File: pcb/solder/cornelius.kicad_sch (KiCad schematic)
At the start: 116 parts, among them J1 AVR-ISP-6, SW1 SW_Push, U1 ATmega32U4-MU, U2 PRTR5V0U2X, Y1 16MHz

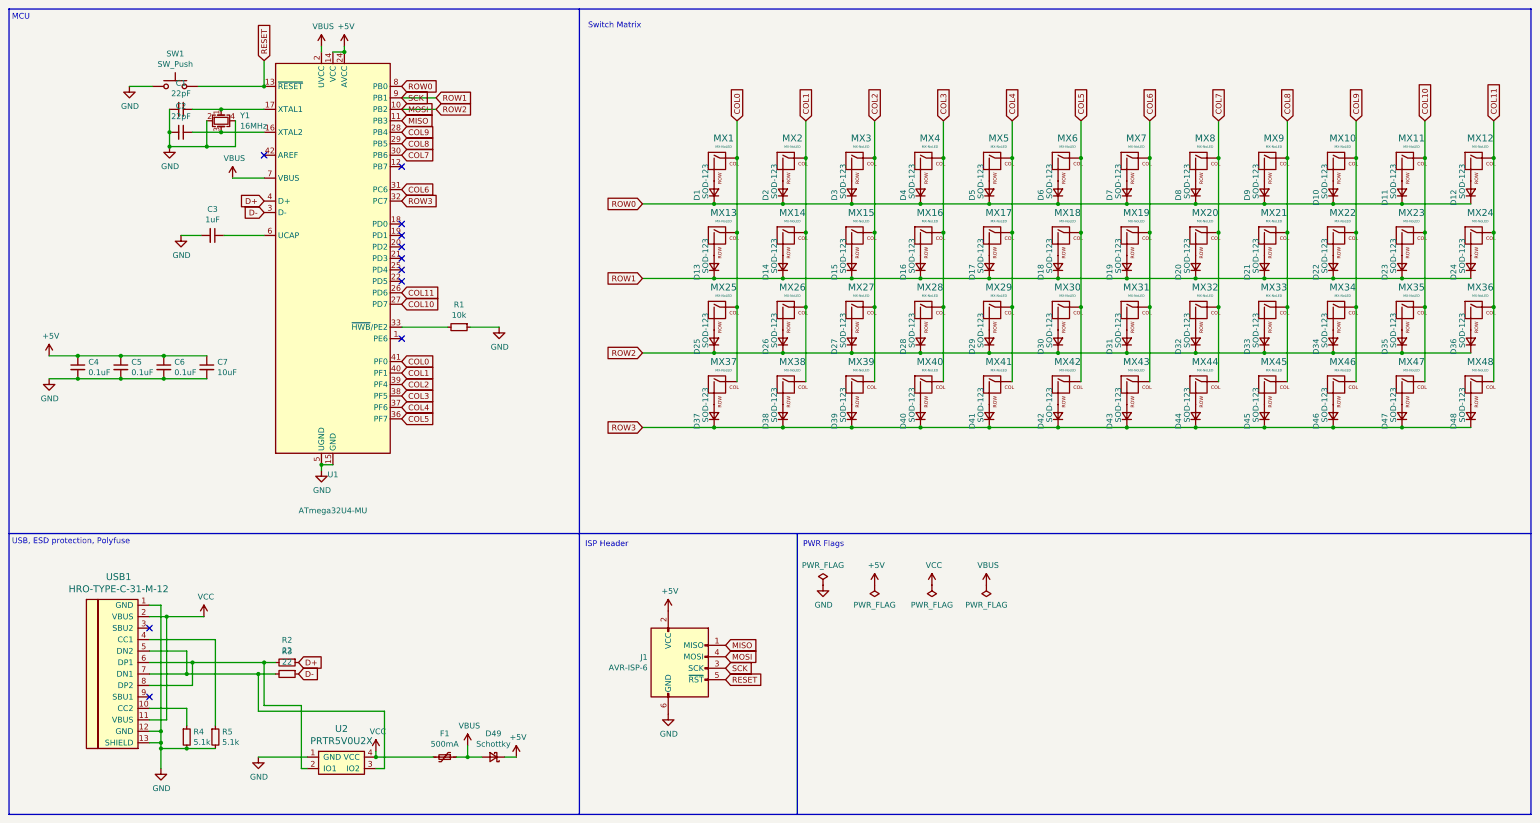
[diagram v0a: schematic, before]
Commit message: Add solder pcb
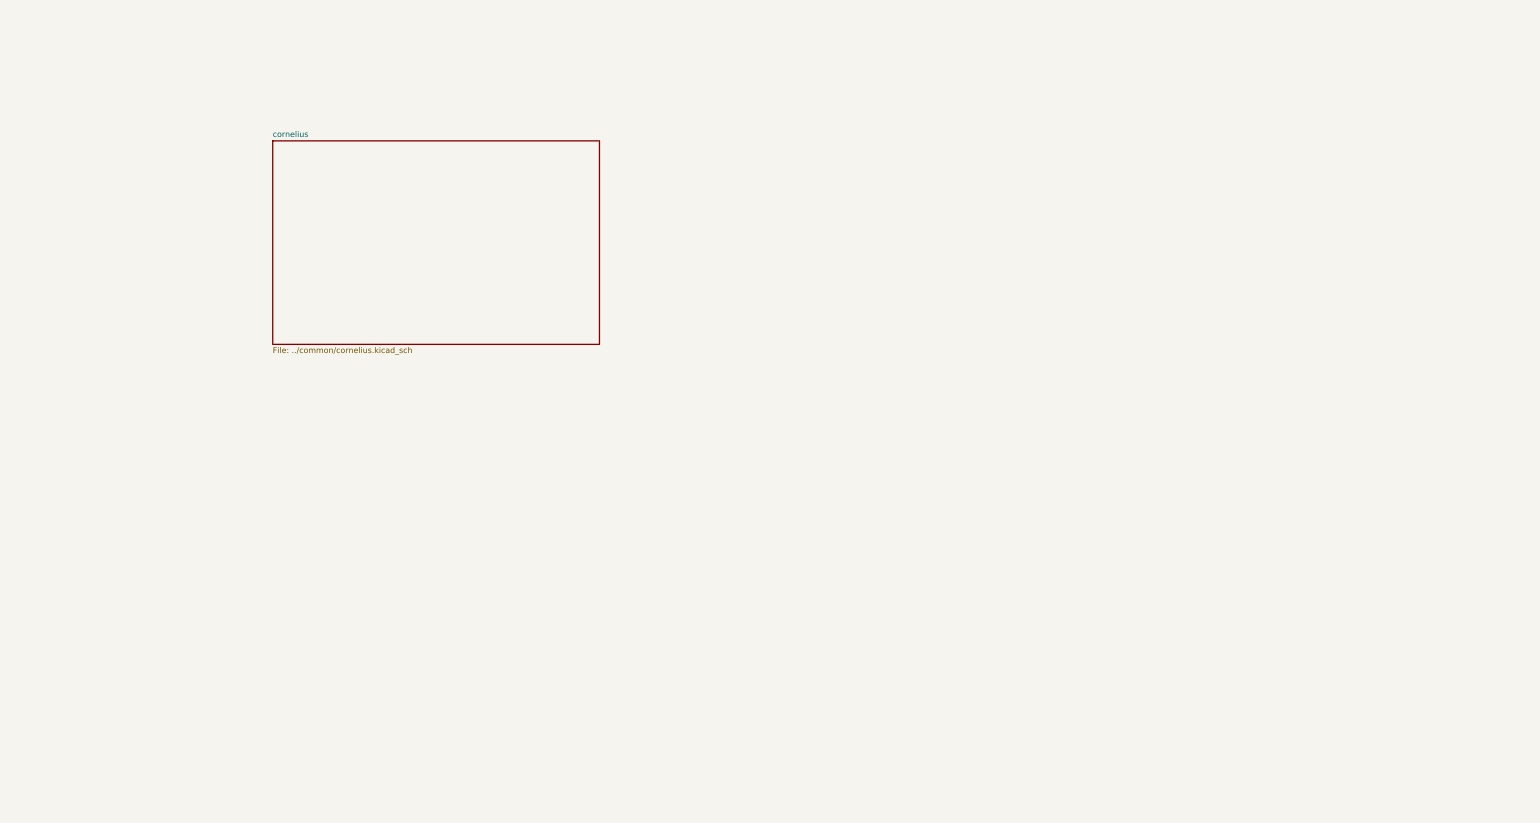
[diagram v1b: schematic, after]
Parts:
- removed C1, C2: 22pF, Capacitor_SMD:C_0603_1608Metric, symbol Device:C_Small
- removed C3: 1uF, Capacitor_SMD:C_0603_1608Metric, symbol Device:C_Small
- removed C4, C5, C6: 0.1uF, Capacitor_SMD:C_0603_1608Metric, symbol Device:C_Small
- removed C7: 10uF, Capacitor_SMD:C_0603_1608Metric, symbol Device:C_Small
- removed D1, D10, D11, D12, D13, D14, D15, D16, D17, D18, D19, D2, D20, D21, D22, D23, D24, D25, D26, D27, D28, D29, D3, D30, D31, D32, D33, D34, D35, D36, D37, D38, D39, D4, D40, D41, D42, D43, D44, D45, D46, D47, D48, D5, D6, D7, D8, D9: SOD-123, Diode_SMD:D_SOD-123, symbol Device:D_Small
- removed D49: Schottky, Diode_SMD:D_SOD-123, symbol Device:D_Schottky_Small
- removed F1: 500mA, Fuse:Fuse_1206_3216Metric, symbol Device:Polyfuse_Small
- removed J1: AVR-ISP-6, Molex-0548190589:Reset_Pretty-Mask, symbol cornelius-rescue:AVR-ISP-6-Connector
- removed MX1, MX10, MX11, MX12, MX13, MX14, MX15, MX16, MX17, MX18, MX19, MX2, MX20, MX21, MX22, MX23, MX24, MX25, MX26, MX27, MX28, MX29, MX3, MX30, MX31, MX32, MX33, MX34, MX35, MX36, MX37, MX38, MX39, MX4, MX40, MX41, MX42, MX43, MX44, MX45, MX46, MX47, MX48, MX5, MX6, MX7, MX8, MX9: MX-NoLED, MX_Only:MXOnly-1U-Hotswap, symbol MX_Alps_Hybrid:MX-NoLED
- removed R1: 10k, Resistor_SMD:R_0805_2012Metric, symbol Device:R_Small
- removed R2, R3: 22, Resistor_SMD:R_0805_2012Metric, symbol Device:R_Small
- removed R4, R5: 5.1k, Resistor_SMD:R_0805_2012Metric, symbol Device:R_Small
- removed SW1: SW_Push, locallib:SKQGADE010, symbol Switch:SW_Push
- removed U1: ATmega32U4-MU, Housings_DFN_QFN:QFN-44-1EP_7x7mm_Pitch0.5mm, symbol cornelius-rescue:ATmega32U4-MU-MCU_Microchip_ATmega-Orbit-rescue-corne-plus-res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
- removed U2: PRTR5V0U2X, locallib:SOT143B, symbol cornelius-rescue:PRTR5V0U2X-ai03-locallib
- removed USB1: HRO-TYPE-C-31-M-12, Type-C:HRO-TYPE-C-31-M-12-Assembly, symbol cornelius-rescue:HRO-TYPE-C-31-M-12-Type-C
- removed Y1: 16MHz, Crystal:Crystal_SMD_3225-4Pin_3.2x2.5mm, symbol cornelius-rescue:Crystal_GND24_Small-Device-Orbit-rescue-corne-plus-rescue
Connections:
- no-connect marks 11 -> 0
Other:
- added sheet cornelius (../common/cornelius.kicad_sch)
- note removed: "ISP Header"
- note removed: "MCU"
- note removed: "PWR Flags"
- note removed: "Switch Matrix"
- note removed: "USB, ESD protection, Polyfuse"
